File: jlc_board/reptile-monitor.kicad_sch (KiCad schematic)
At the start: 45 parts, among them J1 USB_C_Receptacle_USB2.0, J2 AC_IN, J3 Conn_01x08, J7 LOAD1, J8 LOAD2, K1 ALDP105W, K2 ALDP105W, SW1 RST, SW2 BOOT, U1 ESP32-S2-WROVER, U2 TPS2112PW, U3 AP2112K-3.3, U4 MDC3105LT1G, U5 MDC3105LT1G, Y1 32.768KHz 12.5p

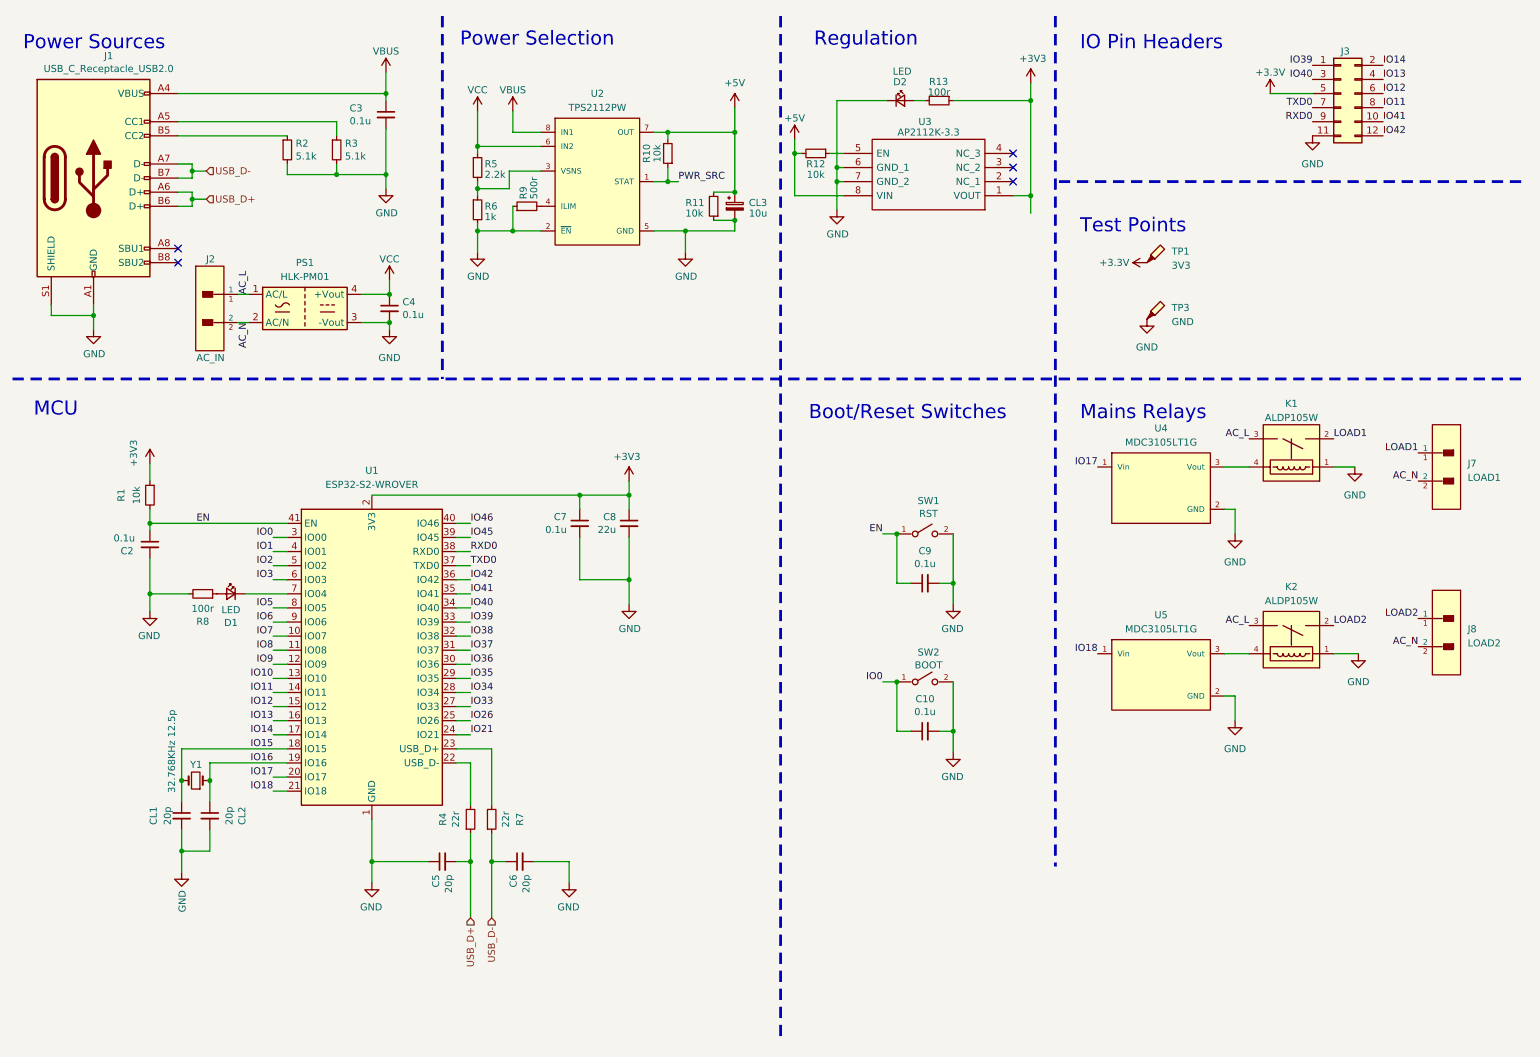
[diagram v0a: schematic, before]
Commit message: rev2
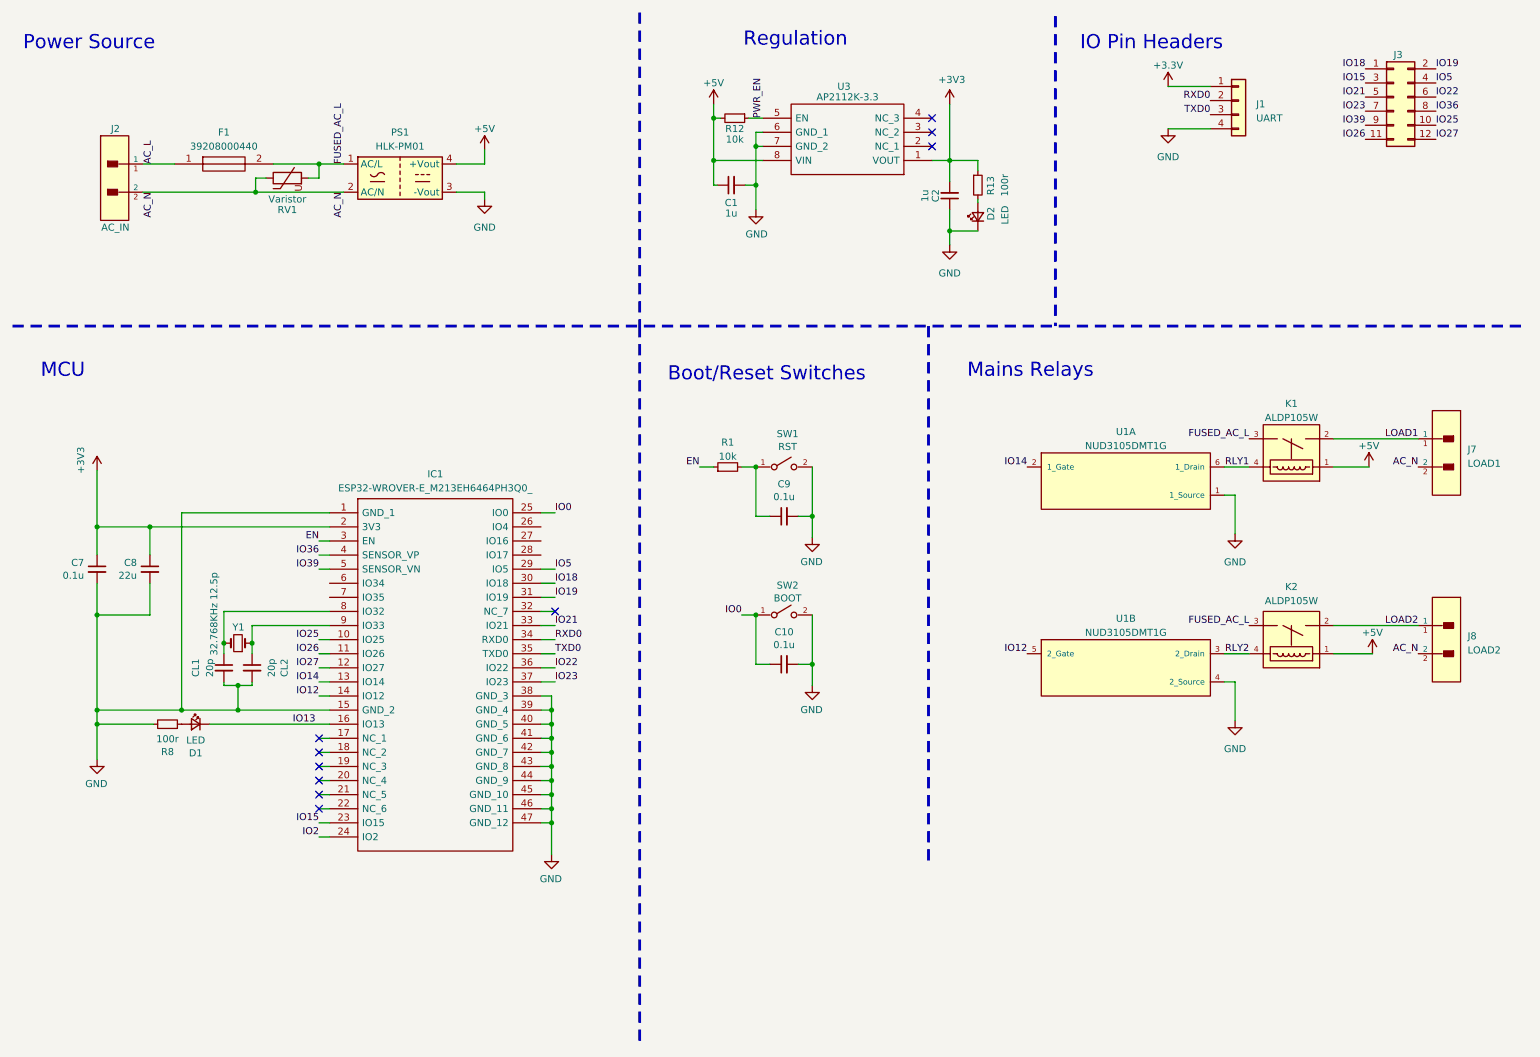
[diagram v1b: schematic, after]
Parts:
- removed C3, C4: 0.1u, Capacitor_SMD:C_0603_1608Metric, symbol Device:C_Small
- removed C5, C6: 20p, Capacitor_SMD:C_0603_1608Metric, symbol Device:C_Small
- removed CL3: 10u, Capacitor_SMD:C_0603_1608Metric, symbol Device:C_Polarized_Small
- removed J1: USB_C_Receptacle_USB2.0, Reptile_Monitor:USB_C_Receptacle_HRO_TYPE-C-31-M-12, symbol Connector:USB_C_Receptacle_USB2.0
- removed R10, R11: 10k, Resistor_SMD:R_0603_1608Metric, symbol Device:R_Small
- removed R2, R3: 5.1k, Resistor_SMD:R_0603_1608Metric, symbol Device:R_Small
- removed R4, R7: 22r, Resistor_SMD:R_0603_1608Metric, symbol Device:R_Small
- removed R5: 2.2k, Resistor_SMD:R_0603_1608Metric, symbol Device:R_Small
- removed R6: 1k, Resistor_SMD:R_0603_1608Metric, symbol Device:R_Small
- removed R9: 500r, Resistor_SMD:R_0603_1608Metric, symbol Device:R_Small
- removed TP1: 3V3, TestPoint:TestPoint_THTPad_1.0x1.0mm_Drill0.5mm, symbol Connector:TestPoint_Probe
- removed TP3: GND, TestPoint:TestPoint_THTPad_1.0x1.0mm_Drill0.5mm, symbol Connector:TestPoint_Probe
- removed U1: ESP32-S2-WROVER, RF_Module:ESP32-S2-WROVER, symbol RF_Module:ESP32-S2-WROVER
- removed U2: TPS2112PW, Reptile_Monitor:Texas_Instruments-TPS2112PW, symbol Reptile_Monitor:TPS2112PW
- removed U4, U5: MDC3105LT1G, Reptile_Monitor:ON_Semiconductor-318-08-01_2018-AS, symbol Reptile_Monitor:MDC3105LT1G
- added C1: 1u, Capacitor_SMD:C_0805_2012Metric, symbol Device:C_Small
- added F1: 39208000440, SamacSys_Parts:TO508P400X850X850-2P, symbol SamacSys_Parts:39215000000
- added IC1: ESP32-WROVER-E_M213EH6464PH3Q0_, SamacSys_Parts:ESP32WROVEREM213EH6464PH3Q0, symbol SamacSys_Parts:ESP32-WROVER-E_M213EH6464PH3Q0_
- added J1: UART, Connector_PinHeader_2.54mm:PinHeader_1x04_P2.54mm_Vertical, symbol Connector_Generic:Conn_01x04
- added RV1: Varistor, Varistor:RV_Disc_D7mm_W3.4mm_P5mm, symbol Device:Varistor
- added U1: NUD3105DMT1G, reptile-monitor:ON_Semi-318F-0-0-0, symbol Reptile_Monitor:NUD3105DMT1G
- C2: value 0.1u -> 1u; footprint Capacitor_SMD:C_0603_1608Metric -> Capacitor_SMD:C_0805_2012Metric; LCSC C14663 -> (none); Series (none) -> X7R or X5R
- R1: LCSC C99198 -> (none)
- Y1: footprint Reptile_Monitor:Crystal_SMD_3215-2Pin_3.2x1.5mm -> reptile-monitor:Crystal_SMD_3215-2Pin_3.2x1.5mm
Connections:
- net IO11 is gone; now on net IO36: J3.8 (Pin_8)
- net IO40 is gone; now on net IO15: J3.3 (Pin_3)
- net VCC is gone; now on net +5V: PS1.4 (+Vout)
- net +3V3: now also C2.2, IC1.2 (3V3), J1.1 (Pin_1); no longer J3.5 (Pin_5), R1.1
- net +5V: now also K1.1, K2.1, C1.1
- net AC_L: now also F1.1; no longer K1.3 (COM), K2.3 (COM), PS1.1 (AC/L)
- net AC_N: now also RV1.1
- net EN: now also R1.1, IC1.3 (EN); no longer C2.1, C9.1, R1.2, SW1.1
- net GND: now also C2.1, C1.2, IC1.1 (GND_1), IC1.15 (GND_2), IC1.38 (GND_3), IC1.39 (GND_4), IC1.40 (GND_5), IC1.41 (GND_6), IC1.42 (GND_7), IC1.43 (GND_8), IC1.44 (GND_9), IC1.45 (GND_10), IC1.46 (GND_11), IC1.47 (GND_12), J1.4 (Pin_4), U1.1 (1_Source), U1.4 (2_Source); no longer C2.2, J3.11 (Pin_11), K1.1, K2.1
- net IO0: now also IC1.25 (IO0)
- net IO12: now also IC1.14 (IO12), U1.5 (2_Gate); no longer J3.6 (Pin_6)
- net IO13: now also D1.1 (K), IC1.16 (IO13); no longer J3.4 (Pin_4)
- net IO14: now also IC1.13 (IO14), U1.2 (1_Gate); no longer J3.2 (Pin_2)
- net IO15: now also IC1.23 (IO15); no longer CL1.1, Y1.2
- net IO18: now also J3.1 (Pin_1), IC1.30 (IO18)
- net IO2: now also IC1.24 (IO2)
- net IO21: now also J3.5 (Pin_5), IC1.33 (IO21)
- net IO26: now also J3.11 (Pin_11), IC1.11 (IO26)
- net IO36: now also IC1.4 (SENSOR_VP)
- net IO39: now also J3.9 (Pin_9), IC1.5 (SENSOR_VN); no longer J3.1 (Pin_1)
- net IO5: now also J3.4 (Pin_4), IC1.29 (IO5)
- net RXD0: now also IC1.34 (RXD0), J1.2 (Pin_2); no longer J3.9 (Pin_9)
- net TXD0: now also IC1.35 (TXD0), J1.3 (Pin_3); no longer J3.7 (Pin_7)
- net PWR_EN: now reaches R12.1, U3.5 (EN)
- net RLY1: now reaches K1.4
- net RLY1: now also U1.6 (1_Drain)
- net RLY2: now reaches K2.4
- net RLY2: now also U1.3 (2_Drain)
- net IO16: no longer names the net of CL2.1, Y1.1
- net IO16: now also IC1.9 (IO33)
- net IO41 renamed IO25
- net IO25: now also IC1.10 (IO25)
- net IO42 renamed IO27
- net IO27: now also IC1.12 (IO27)
- new net: C9.1, R1.2, SW1.1
- new net: CL1.1, IC1.8 (IO32), Y1.2
- new net FUSED_AC_L: F1.2, K1.3 (COM), K2.3 (COM), PS1.1 (AC/L), RV1.2
- new net IO19: IC1.31 (IO19), J3.2 (Pin_2)
- new net IO22: IC1.36 (IO22), J3.6 (Pin_6)
- new net IO23: IC1.37 (IO23), J3.7 (Pin_7)
- no-connect marks 5 -> 10
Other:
- note added: "Power Source"
- note removed: "Power Selection"
- note removed: "Power Sources"
- note removed: "Test Points"
- moved on the sheet: C10, C7, C8, C9, D1, D2, J2, J3, J7, J8, PS1, R12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
